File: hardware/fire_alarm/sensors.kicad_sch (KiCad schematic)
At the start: 2 parts, among them U5 DS18B20

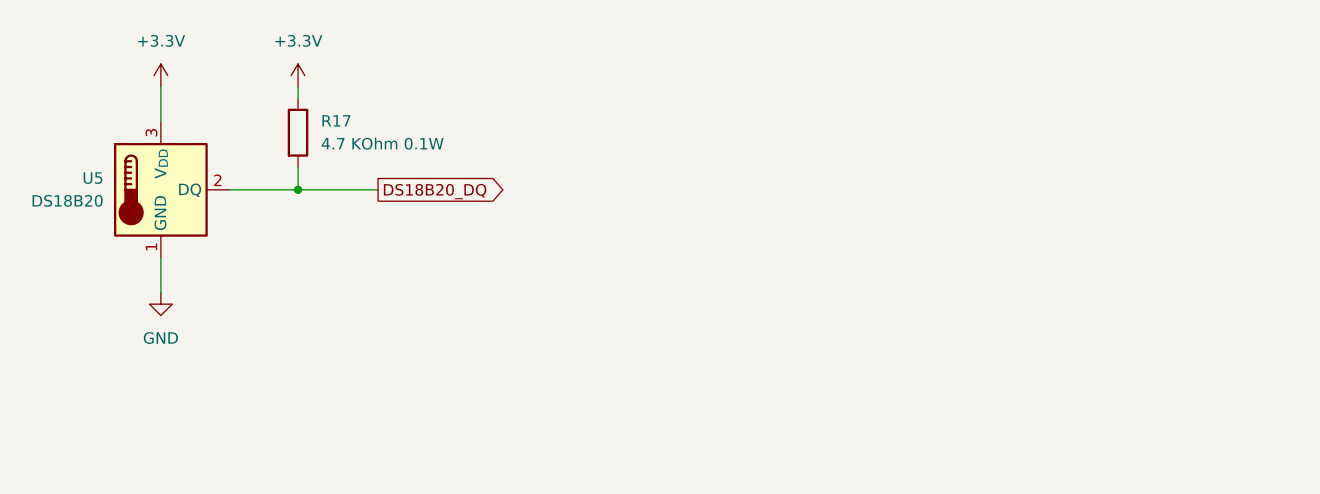
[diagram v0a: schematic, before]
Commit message: feat: complete schematic
Signed-off-by: Trung Hieu Nguyen <hieu.nguyenarc03@gmail.com>
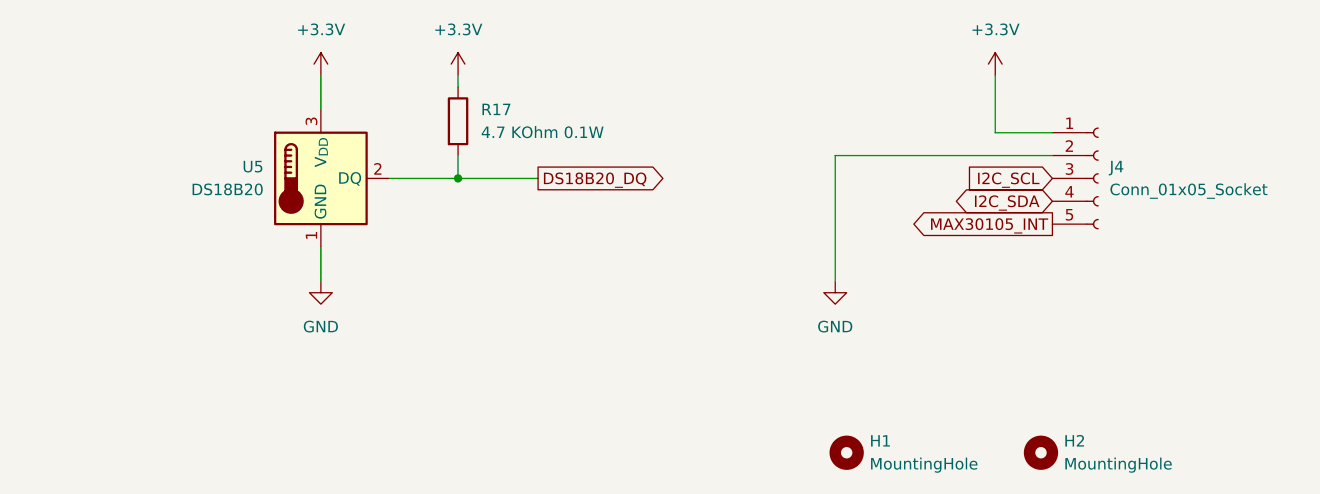
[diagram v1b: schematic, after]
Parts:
- added H1, H2: MountingHole, MountingHole:MountingHole_3.2mm_M3, symbol Mechanical:MountingHole
- added J4: Conn_01x05_Socket, Connector_PinSocket_2.54mm:PinSocket_1x05_P2.54mm_Vertical, symbol Connector:Conn_01x05_Socket
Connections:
- net +3.3V: now also J4.1 (Pin_1)
- net GND: now also J4.2 (Pin_2)
- new net I2C_SCL: J4.3 (Pin_3)
- new net I2C_SDA: J4.4 (Pin_4)
- new net MAX30105_INT: J4.5 (Pin_5)
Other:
- moved on the sheet: R17, U5
